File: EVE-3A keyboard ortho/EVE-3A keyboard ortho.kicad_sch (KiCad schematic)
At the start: 128 parts, among them J1 Conn_01x04_Male, J2 Conn_01x06_Male, SW1 1, SW10 W, SW11 S, SW12 X, SW13 4, SW14 E, SW15 D, SW16 C, SW17 5, SW18 R, SW19 F, SW2 Esc, SW20 V, SW21 6, SW22 T, SW23 G, SW24 B, SW25 Space, SW26 7, SW27 Y, SW28 H, SW29 N, SW3 Ctrl, SW30 Space, SW31 8, SW32 U, SW33 J, SW34 M, SW35 Space, SW36 9, SW37 I, SW38 K, SW39 ,, SW4 ShiftL, SW40 0, SW41 O, SW42 L, SW43 ., SW44 :, SW45 P, SW46 ;, SW47 /, SW48 - =, SW49 LineFeed, SW5 2, SW50 @, SW51 ShiftR, SW52 [, SW53 Enter, SW54 \, SW55 ], SW56 _ Rub, SW57 Repeat, SW58 ^ ~ Home, SW59 Here Is, SW6 Q, SW60 Break, SW61 Clear, SW62 Special, SW7 A, SW8 Z, SW9 3, U1 74LS138, U2 74LS138

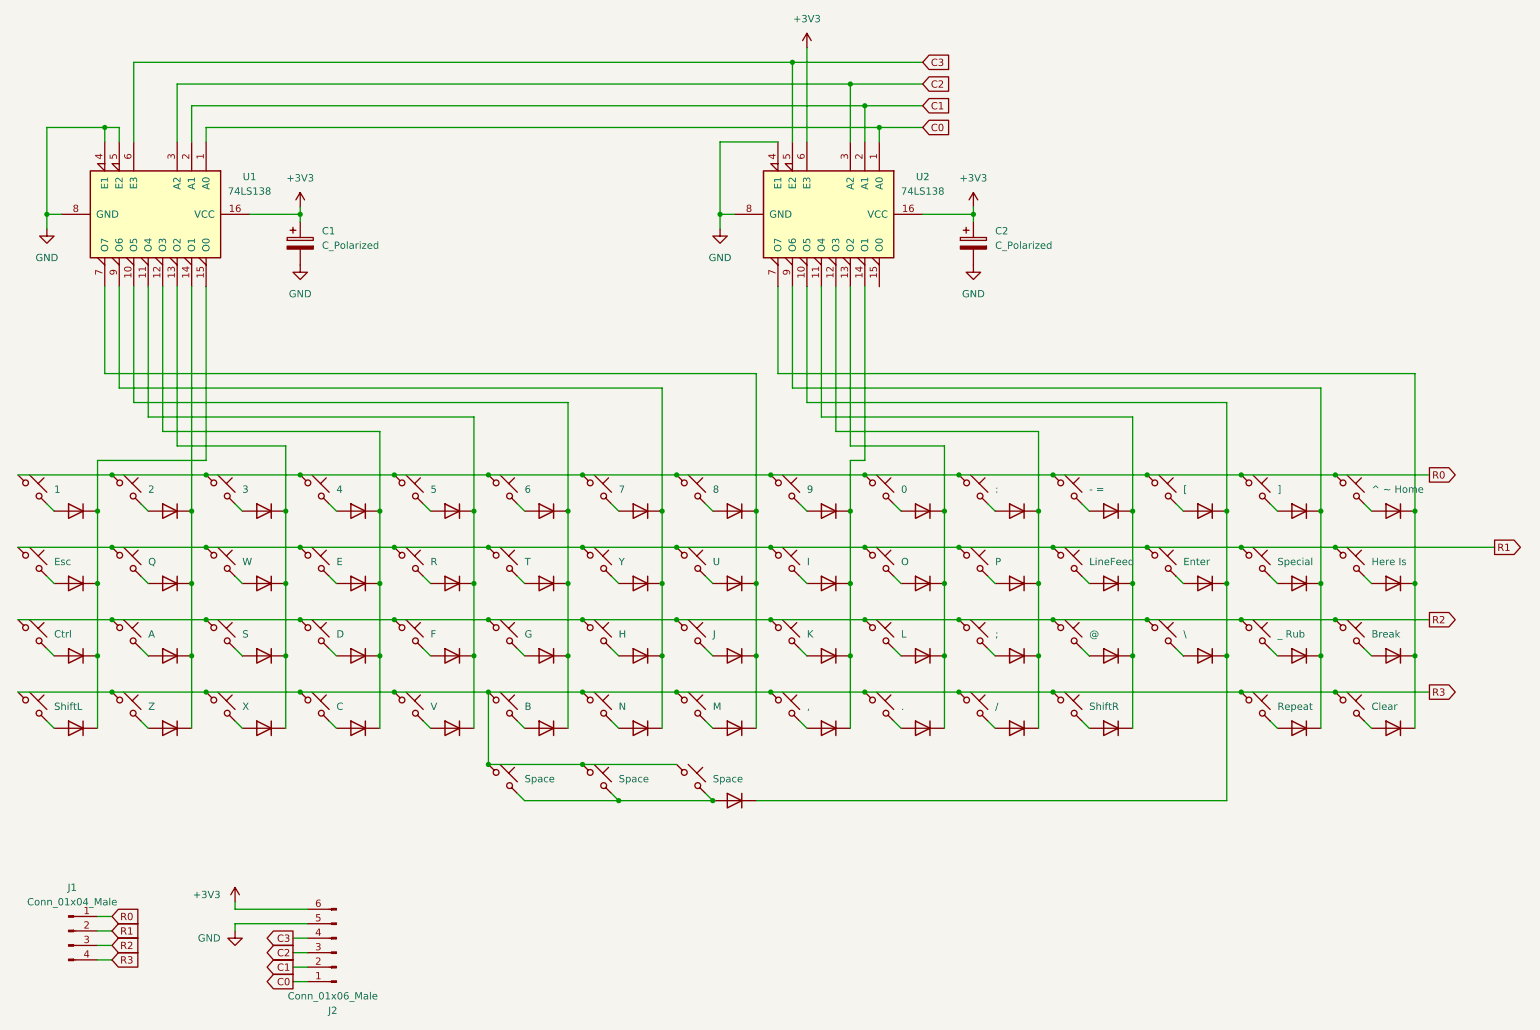
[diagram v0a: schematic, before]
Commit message: interim checkin
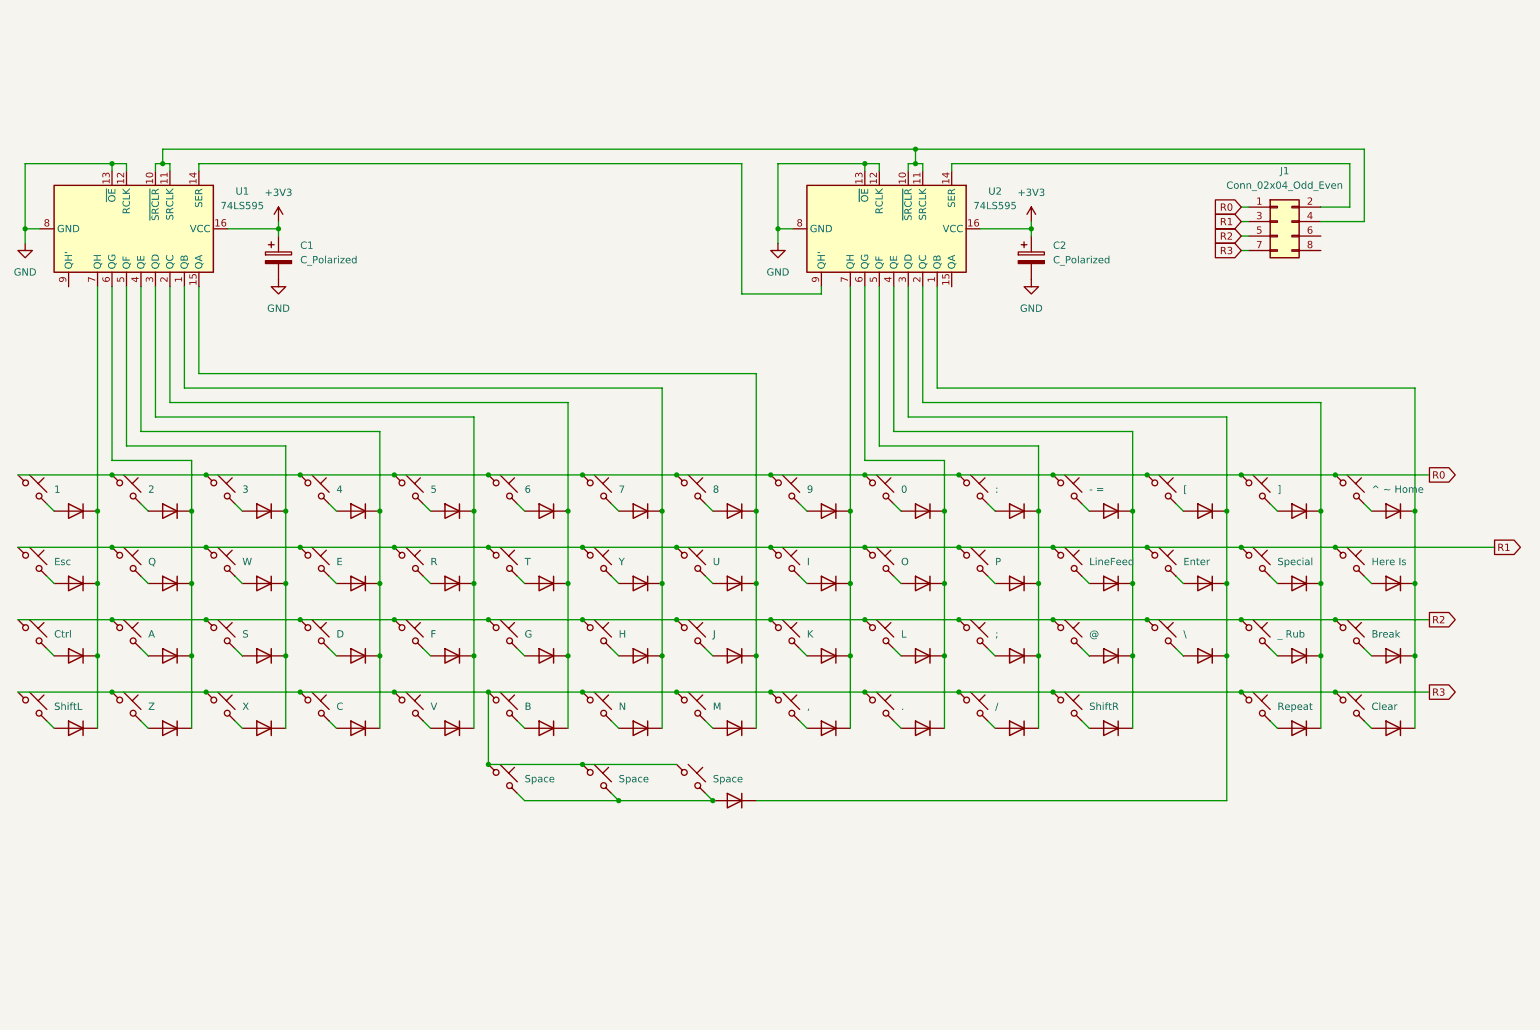
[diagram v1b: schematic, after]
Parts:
- removed J1: Conn_01x04_Male, Connector_PinHeader_2.54mm:PinHeader_1x04_P2.54mm_Horizontal, symbol Connector:Conn_01x04_Male
- removed J2: Conn_01x06_Male, Connector_PinHeader_2.54mm:PinHeader_1x06_P2.54mm_Horizontal, symbol Connector:Conn_01x06_Male
- removed U1, U2: 74LS138, Package_DIP:DIP-16_W7.62mm_Socket, symbol 74xx:74LS138
- added J1: Conn_02x04_Odd_Even, Connector_IDC:IDC-Header_2x04_P2.54mm_Vertical, symbol Connector_Generic:Conn_02x04_Odd_Even
- added U1, U2: 74LS595, Package_DIP:DIP-16_W7.62mm_Socket, symbol 74xx:74LS595
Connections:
- net +3V3: now also U1.16 (VCC), U2.16 (VCC)
- net GND: now also U1.12 (RCLK), U1.13 (~{OE}), U1.8 (GND), U2.12 (RCLK), U2.13 (~{OE}), U2.8 (GND)
- net R0: now also J1.1 (Pin_1)
- net R1: now also J1.3 (Pin_3)
- net R2: now also J1.5 (Pin_5)
- net R3: now also J1.7 (Pin_7)
- net at D53.1 (K), D54.1 (K), D55.1 (K)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: now also U2.2 (QC)
- net at D33.1 (K), D50.1 (K), D51.1 (K)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: now also U2.3 (QD)
- net at D42.1 (K), D43.1 (K), D44.1 (K)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: now also U2.5 (QF)
- net at D5.1 (K), D6.1 (K), D7.1 (K)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: now also U1.6 (QG)
- net at D29.1 (K), D30.1 (K), D31.1 (K)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: now also U1.15 (QA)
- net at D38.1 (K), D39.1 (K), D40.1 (K)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: now also U2.6 (QG)
- net at D1.1 (K), D2.1 (K), D3.1 (K)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: now also U1.7 (QH)
- net at D10.1 (K), D11.1 (K), D12.1 (K)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: now also U1.5 (QF)
- net at D17.1 (K), D18.1 (K), D19.1 (K)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: now also U1.3 (QD)
- net at D13.1 (K), D14.1 (K), D15.1 (K)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: now also U1.4 (QE)
- net at D25.1 (K), D26.1 (K), D27.1 (K)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: now also U1.1 (QB)
- net at D34.1 (K), D35.1 (K), D36.1 (K)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: now also U2.7 (QH)
- net at D56.1 (K), D57.1 (K), D58.1 (K)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: now also U2.1 (QB)
- net at D46.1 (K), D47.1 (K), D48.1 (K)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: now also U2.4 (QE)
- net at D21.1 (K), D22.1 (K), D23.1 (K)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: now also U1.2 (QC)
- new net: J1.4 (Pin_4), U1.10 (~{SRCLR}), U1.11 (SRCLK), U2.10 (~{SRCLR}), U2.11 (SRCLK)
- new net: U1.14 (SER), U2.9 (QH')
- new net: J1.2 (Pin_2), U2.14 (SER)
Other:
- moved on the sheet: C2
